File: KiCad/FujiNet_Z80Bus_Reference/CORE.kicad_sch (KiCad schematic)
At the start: 23 parts, among them IC1 74244N, IC13 7432N, IC2 7404N, IC3 7474N, IC5 7408N

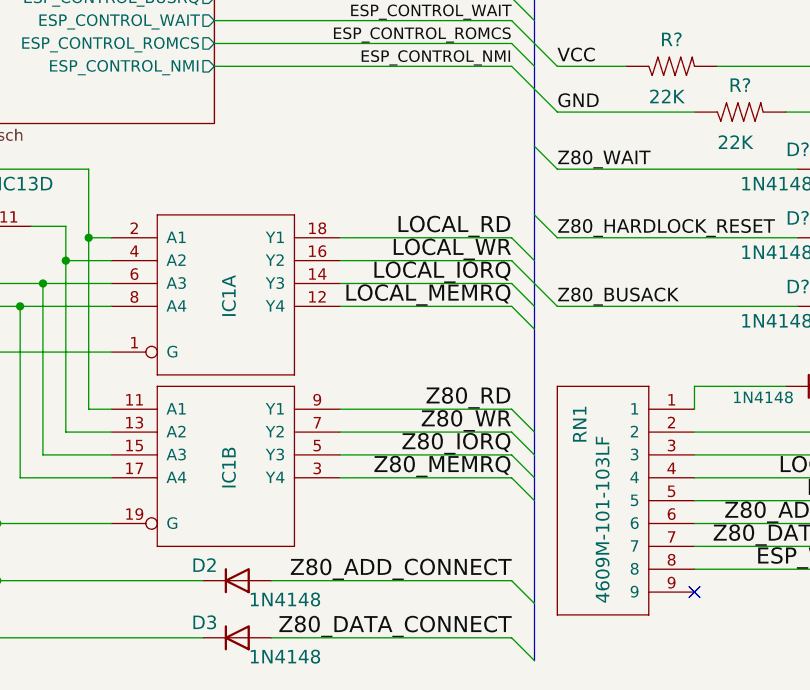
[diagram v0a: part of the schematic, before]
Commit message: Single PCB layout experiements
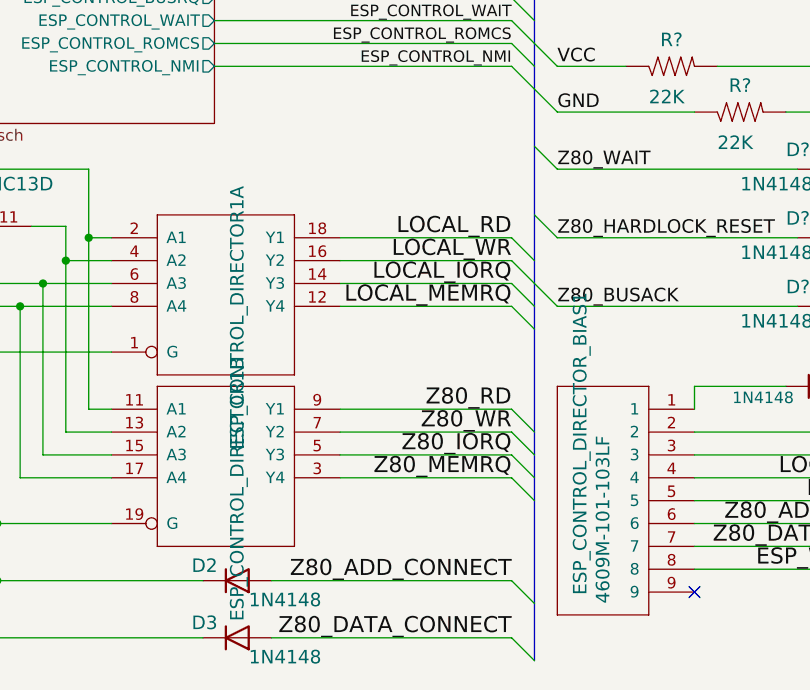
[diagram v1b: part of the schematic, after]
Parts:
- renumbered IC1 to ESP_CONTROL_DIRECTOR1, RN1 to ESP_CONTROL_DIRECTOR_BIAS1
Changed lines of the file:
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@@
   (symbol (lib_id "FujiNet_Z80Bus_Reference-rescue:4609M-101-103LF-Z80ESP-eagle-import") (at 140.97 167.64 0) (mirror y) (unit 1)
     (in_bom yes) (on_board yes) (dnp no)
-    (property "Reference" "RN1" (at 128.27 171.45 90)
-      (effects (font (size 1.4986 1.4986)) (justify left))
+    (property "Reference" "ESP_CONTROL_DIRECTOR_BIAS1" (at 128.27 171.45 90)
+      (effects (font (size 1.4986 1.4986)))
     )
     (property "Value" "4609M-101-103LF" (at 130.81 189.23 90)
@@
       (project "FujiNet_Z80Bus_Reference"
         (path "/532c0392-800e-45cc-8170-6d32f2390e83/00000000-0000-0000-0000-000068f578e9"
-          (reference "RN1") (unit 1)
+          (reference "ESP_CONTROL_DIRECTOR_BIAS1") (unit 1)
         )
         (path "/532c0392-800e-45cc-8170-6d32f2390e83/00000000-0000-0000-0000-000068f578e9/00000000-0000-0000-0000-000068fd7452"
@@
   (symbol (lib_id "FujiNet_Z80Bus_Reference-rescue:74244N-Z80ESP-eagle-import") (at 88.9 153.67 0) (unit 1)
     (in_bom yes) (on_board yes) (dnp no)
-    (property "Reference" "IC1" (at 90.17 157.48 90)
-      (effects (font (size 1.4986 1.4986)) (justify left bottom))
+    (property "Reference" "ESP_CONTROL_DIRECTOR1" (at 90.17 157.48 90)
+      (effects (font (size 1.4986 1.4986)))
     )
     (property "Value" "74244N" (at 81.28 166.37 0)
@@
       (project "FujiNet_Z80Bus_Reference"
         (path "/532c0392-800e-45cc-8170-6d32f2390e83/00000000-0000-0000-0000-000068f578e9"
-          (reference "IC1") (unit 1)
+          (reference "ESP_CONTROL_DIRECTOR1") (unit 1)
         )
         (path "/532c0392-800e-45cc-8170-6d32f2390e83/00000000-0000-0000-0000-000068f578e9/00000000-0000-0000-0000-000068fd7452"
@@
   (symbol (lib_id "FujiNet_Z80Bus_Reference-rescue:74244N-Z80ESP-eagle-import") (at 88.9 172.72 0) (unit 2)
     (in_bom yes) (on_board yes) (dnp no)
-    (property "Reference" "IC1" (at 90.17 176.53 90)
-      (effects (font (size 1.4986 1.4986)) (justify left bottom))
+    (property "Reference" "ESP_CONTROL_DIRECTOR1" (at 90.17 176.53 90)
+      (effects (font (size 1.4986 1.4986)))
     )
     (property "Value" "74244N" (at 81.28 185.42 0)
@@
       (project "FujiNet_Z80Bus_Reference"
         (path "/532c0392-800e-45cc-8170-6d32f2390e83/00000000-0000-0000-0000-000068f578e9"
-          (reference "IC1") (unit 2)
-        )
-        (path "/532c0392-800e-45cc-8170-6d32f2390e83/00000000-0000-0000-0000-000068f578e9/00000000-0000-0000-0000-000068fd7452"
+          (reference "ESP_CONTROL_DIRECTOR1") (unit 2)
+        )
+        (path "/532c0392-800e-45cc-8170-6d32f2390e83/00000000-0000-0000-0000-000068f578e9/00000000-0000-0000-0000-000068fd7452"

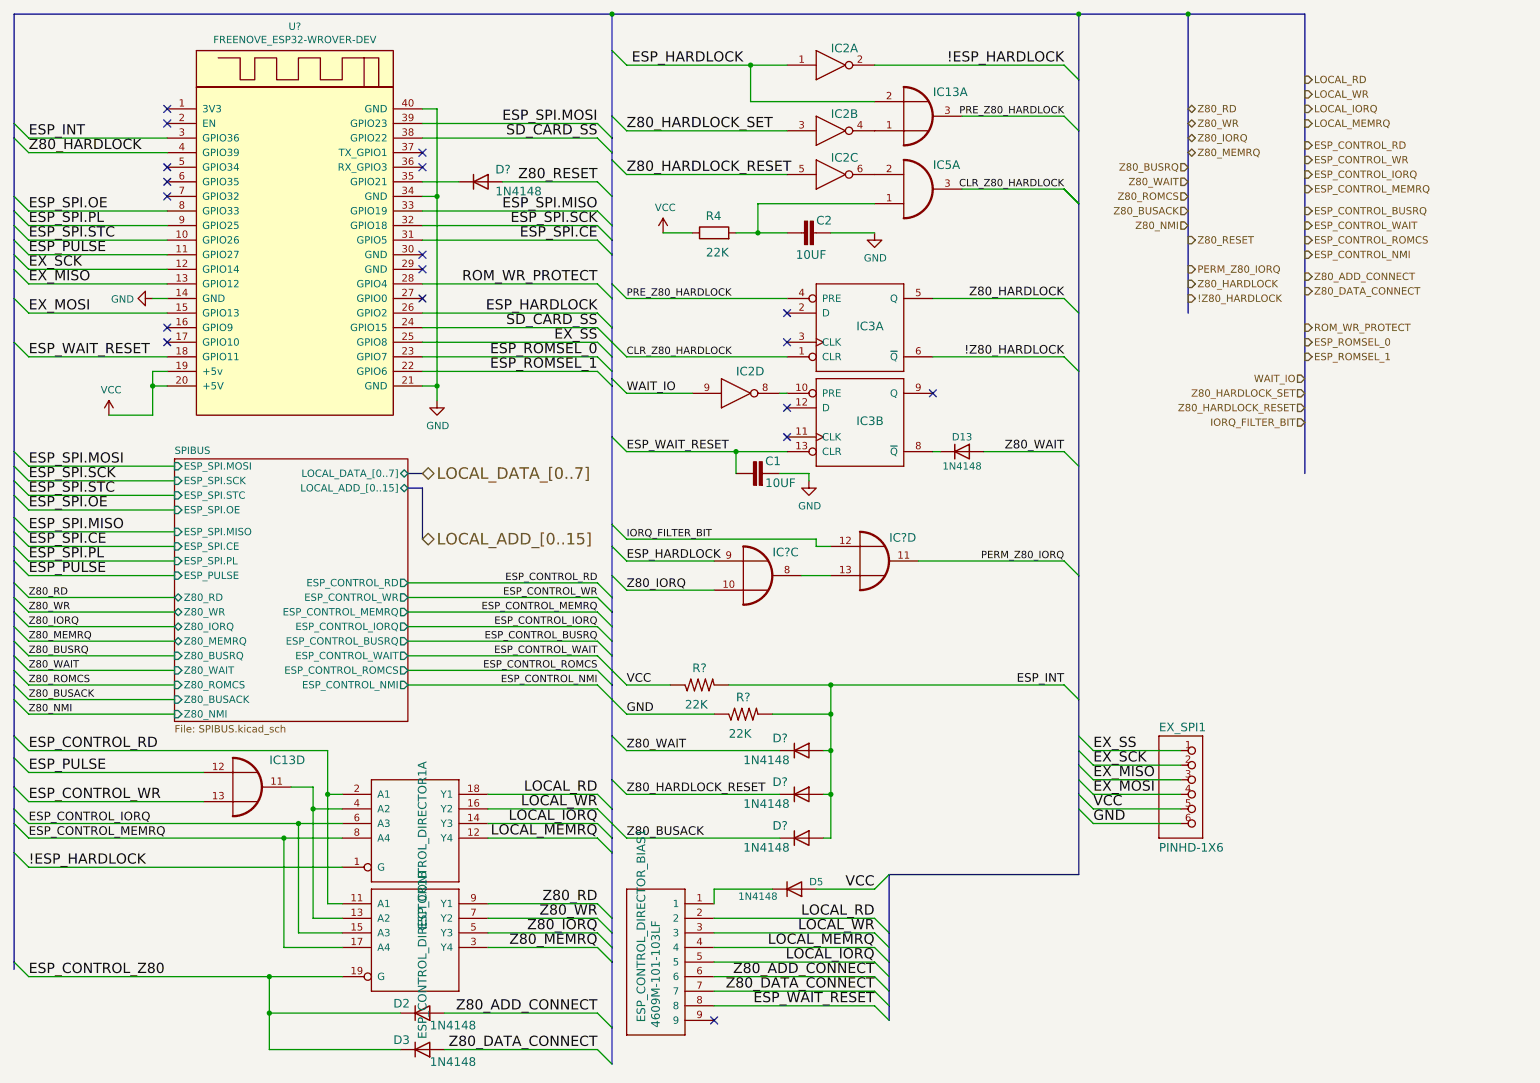
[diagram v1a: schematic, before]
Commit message: Massive fix to KiCad Labels
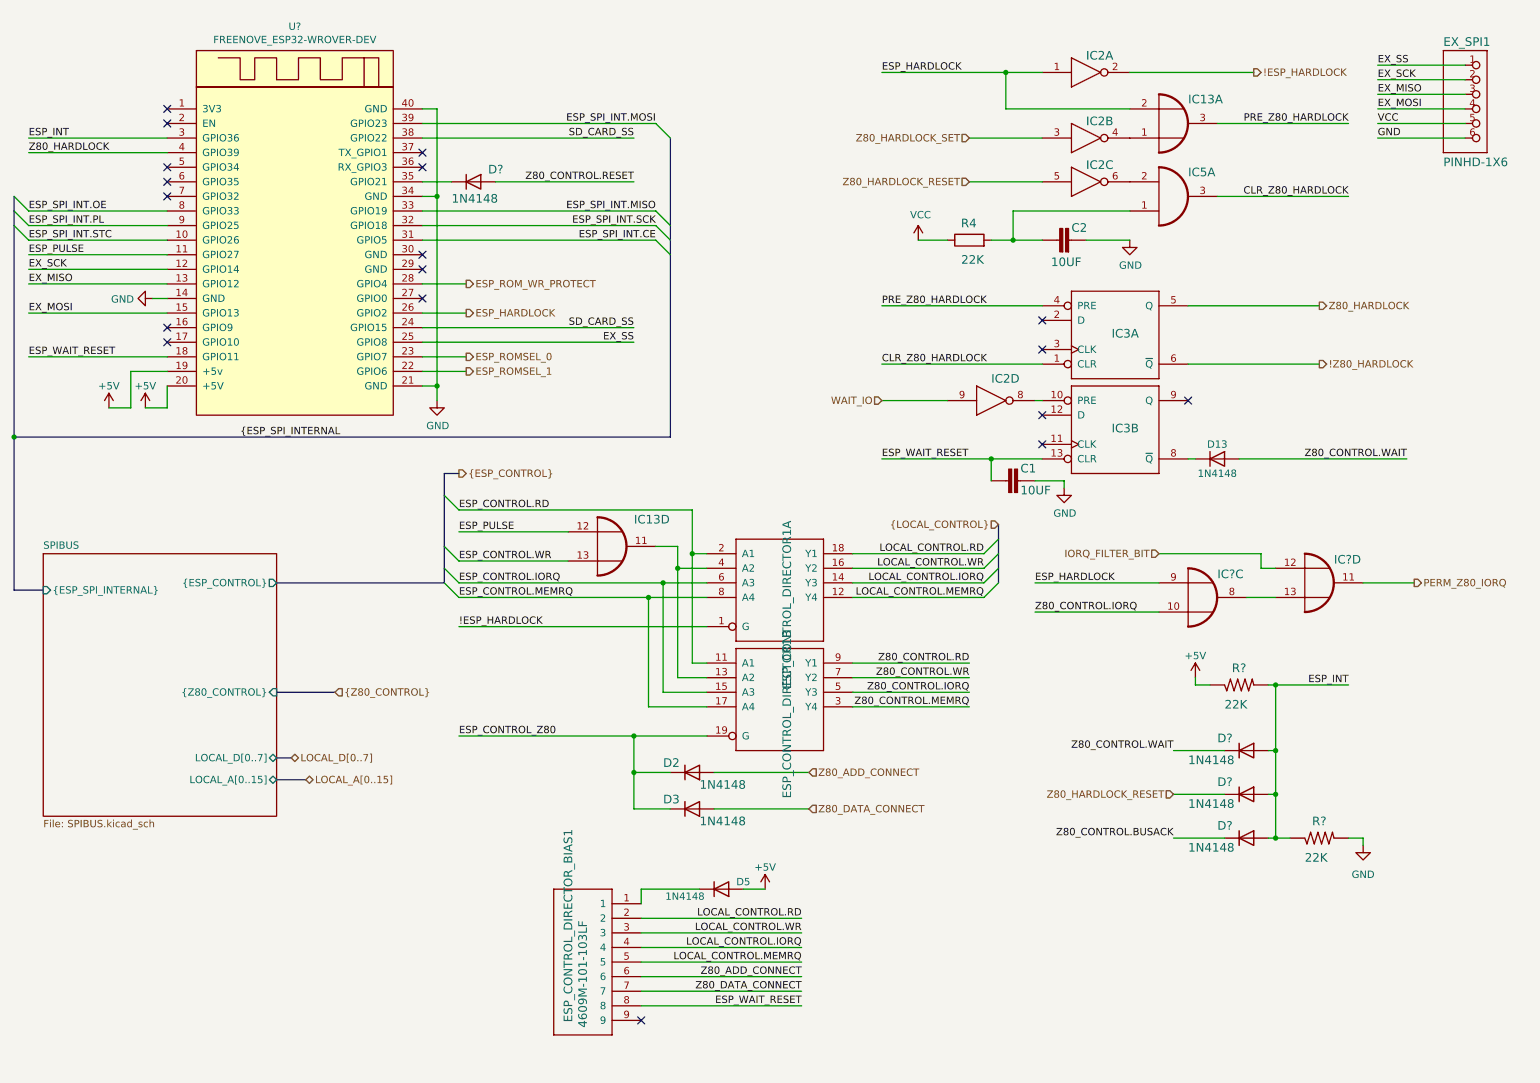
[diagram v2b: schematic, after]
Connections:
- net ESP_INT: now also R?.1; no longer R?.2
- net GND: now also R?.2; no longer R?.1
- net VCC: no longer D5.2 (A), R?.1, U?.19 (+5v), U?.20 (+5V)
- net ESP_CONTROL_IORQ renamed ESP_CONTROL.IORQ
- net ESP_CONTROL_MEMRQ renamed ESP_CONTROL.MEMRQ
- net ESP_CONTROL_RD renamed ESP_CONTROL.RD
- net ESP_CONTROL_WR renamed ESP_CONTROL.WR
- net ESP_SPI.CE renamed ESP_SPI_INT.CE
- net ESP_SPI.MISO renamed ESP_SPI_INT.MISO
- net ESP_SPI.MOSI renamed ESP_SPI_INT.MOSI
- net ESP_SPI.OE renamed ESP_SPI_INT.OE
- net ESP_SPI.PL renamed ESP_SPI_INT.PL
- net ESP_SPI.SCK renamed ESP_SPI_INT.SCK
- net ESP_SPI.STC renamed ESP_SPI_INT.STC
- net LOCAL_IORQ renamed LOCAL_CONTROL.IORQ
- net LOCAL_CONTROL.IORQ: now also ESP_CONTROL_DIRECTOR_BIAS1.4; no longer ESP_CONTROL_DIRECTOR_BIAS1.5
- net LOCAL_MEMRQ renamed LOCAL_CONTROL.MEMRQ
- net LOCAL_CONTROL.MEMRQ: now also ESP_CONTROL_DIRECTOR_BIAS1.5; no longer ESP_CONTROL_DIRECTOR_BIAS1.4
- net LOCAL_RD renamed LOCAL_CONTROL.RD
- net LOCAL_WR renamed LOCAL_CONTROL.WR
- net ROM_WR_PROTECT renamed ESP_ROM_WR_PROTECT
- net Z80_BUSACK renamed Z80_CONTROL.BUSACK
- net Z80_IORQ renamed Z80_CONTROL.IORQ
- net Z80_MEMRQ renamed Z80_CONTROL.MEMRQ
- net Z80_RD renamed Z80_CONTROL.RD
- net Z80_RESET renamed Z80_CONTROL.RESET
- net Z80_WAIT renamed Z80_CONTROL.WAIT
- net Z80_WR renamed Z80_CONTROL.WR
- new net +5V: D5.2 (A), R?.1, U?.19 (+5v), U?.20 (+5V)
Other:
- sheet SPIBUS ports: added LOCAL_A[0..15], LOCAL_D[0..7], {ESP_CONTROL}, {ESP_SPI_INTERNAL}, {Z80_CONTROL}; removed ESP_CONTROL_BUSRQ, ESP_CONTROL_IORQ, ESP_CONTROL_MEMRQ, ESP_CONTROL_NMI, ESP_CONTROL_RD, ESP_CONTROL_ROMCS, ESP_CONTROL_WAIT, ESP_CONTROL_WR, ESP_PULSE, ESP_SPI.CE, ESP_SPI.MISO, ESP_SPI.MOSI, ESP_SPI.OE, ESP_SPI.PL, ESP_SPI.SCK, ESP_SPI.STC, LOCAL_ADD_[0..15], LOCAL_DATA_[0..7], Z80_BUSACK, Z80_BUSRQ, Z80_IORQ, Z80_MEMRQ, Z80_NMI, Z80_RD, Z80_ROMCS, Z80_WAIT, Z80_WR
- moved on the sheet: C1, C2, D13, D2, D3, D5, D?, ESP_CONTROL_DIRECTOR1A, ESP_CONTROL_DIRECTOR1B, ESP_CONTROL_DIRECTOR_BIAS1, EX_SPI1, IC13A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
